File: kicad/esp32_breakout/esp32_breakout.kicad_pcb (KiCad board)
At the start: 2 copper layers, 70 x 35 mm, 26 parts, among them J1 JST B5B-PH-K-S, J10 JST B6B-PH-K-S, J2 JST B5B-PH-K-S, J3 JST B7B-PH-K-S, J4 XT30U-M, J5 HDR F 2.54MM VERT, J6 HDR F 2.54MM 5-pin VERT, J9 JST B6B-PH-K-S, SW1 SS12D10, U1 ESP32 DEV KIT Module 30-pin, U2 LM2596 Module

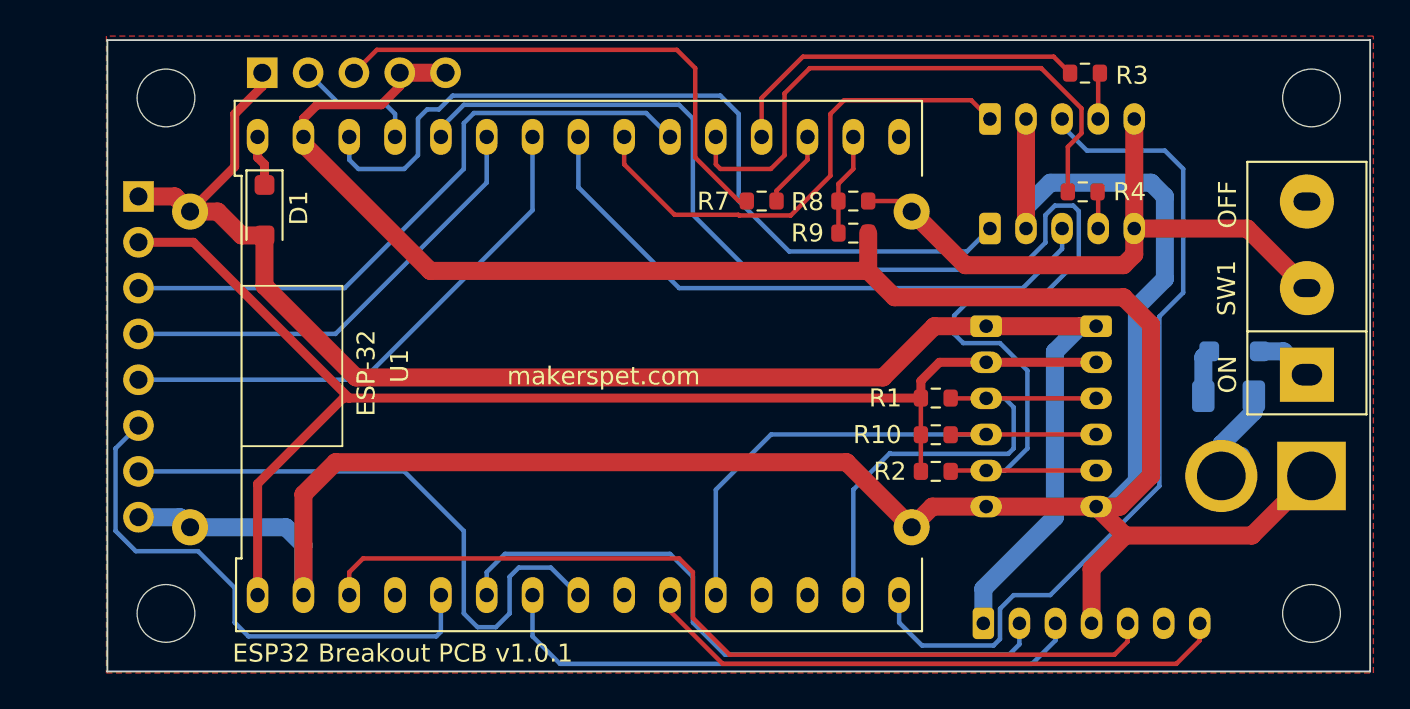
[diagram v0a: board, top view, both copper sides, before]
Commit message: ESP32 PCB v1.1.0
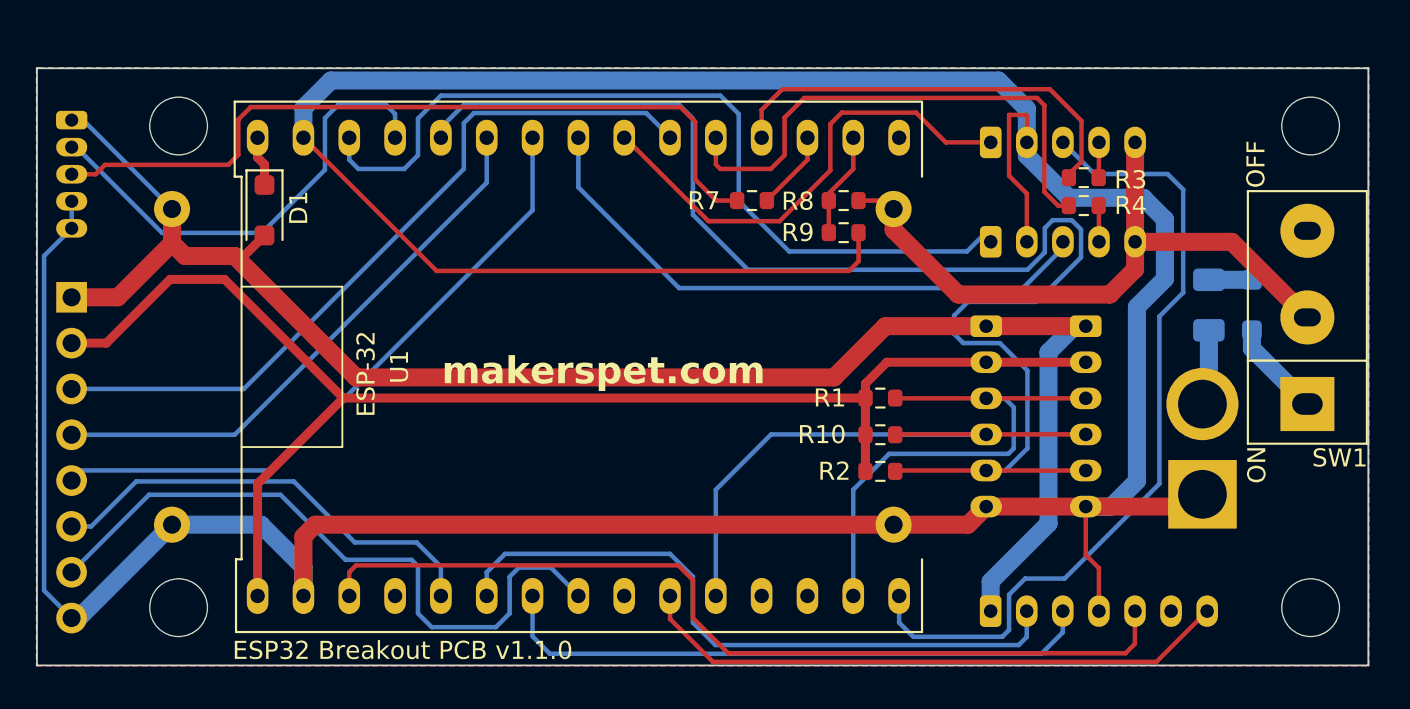
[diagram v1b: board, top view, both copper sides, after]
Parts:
- J5: value HDR F 2.54MM VERT -> HDR 8p M VERT 2.54mm; footprint Connector_PinSocket_2.54mm:PinSocket_1x08_P2.54mm_Vertical -> Connector_PinHeader_2.54mm:PinHeader_1x08_P2.54mm_Vertical
- J6: value HDR F 2.54MM 5-pin VERT -> JST B5B-ZR; footprint Connector_PinSocket_2.54mm:PinSocket_1x05_P2.54mm_Vertical -> Makerspet:JST_ZH_B5B-ZR_1x05_P1.50mm_Vertical
- moved J6 10.9 mm to (123.6, 82.6)
- moved J5 6.71 mm to (123.5, 92.5)
- moved J4 6.13 mm to (186.2, 103.4), turned to 90 degrees
- moved R3 5.79 mm to (179.7, 85.8)
- moved F1 5.17 mm to (186.6, 92.9), turned to 90 degrees
- moved R1 3.07 mm to (168.4, 98.0)
- moved R10 3.07 mm to (168.4, 100.1)
- moved R2 3.07 mm to (168.4, 102.1)
- moved D2 2.74 mm to (189.0, 92.9), turned to 90 degrees
- moved H1 1.71 mm to (129.5, 83.0)
- moved SW1 1.63 mm to (192.0, 93.6)
- moved H2 1.56 mm to (192.2, 83.0)
- moved J2 1.30 mm to (174.5, 83.9)
- moved U2 1.01 mm to (149.1, 96.3)
- moved J3 0.79 mm to (174.5, 109.9)
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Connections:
- net /LDS_MOT_EN renamed /LDS_EN
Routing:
- net GND: track 195.7 -> 221.6 mm
- net /GPIO12_OUT_STRAP: track 7.04 -> 26.0 mm
- net Net-(J6-Pin_3): track 28.7 -> 43.6 mm
- net /GPIO32_TOUCH: track 35.5 -> 41.5 mm
- net /GPIO27_TOUCH: track 25.3 -> 31.3 mm
- net /GPIO26_TOUCH: track 29.8 -> 35.8 mm
- net /GPIO4_TOUCH: track 30.1 -> 25.1 mm
- net /GPIO5_BOOT_STRAP: track 33.8 -> 37.6 mm
- net +3V3: track 75.3 -> 78.7 mm
- net /MOT_FG_LEFT: track 20.6 -> 23.9 mm
- net /MOT_FG_RIGHT: track 32.1 -> 29.3 mm
- net Net-(J4-+): track 6.74 -> 4.24 mm
- net /I2C_SDA: track 30.2 -> 32.7 mm
- net /I2C_SCL: track 27.8 -> 30.3 mm
- net +5V: track 89.3 -> 91.7 mm
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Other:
- board size 70 x 35 mm -> 73.8 x 33.1 mm
- board text added: "+ BATT -"
- board text added: "ESP32 Breakout PCB v1.1.0"
- board text added: "LASER DIST"
- board text added: "LEFT RIGHT"
- board text added: "U.DIST"
- board text removed: "BATT"
- board text removed: "DIST"
- board text removed: "ESP32 Breakout PCB v1.0.1"
- board text removed: "LEFT"
- board text removed: "RIGHT"
